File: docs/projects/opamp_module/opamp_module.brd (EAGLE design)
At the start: 58.1 x 25.4 mm, 12 parts, among them IC1 TL071P, IC2 TL072P

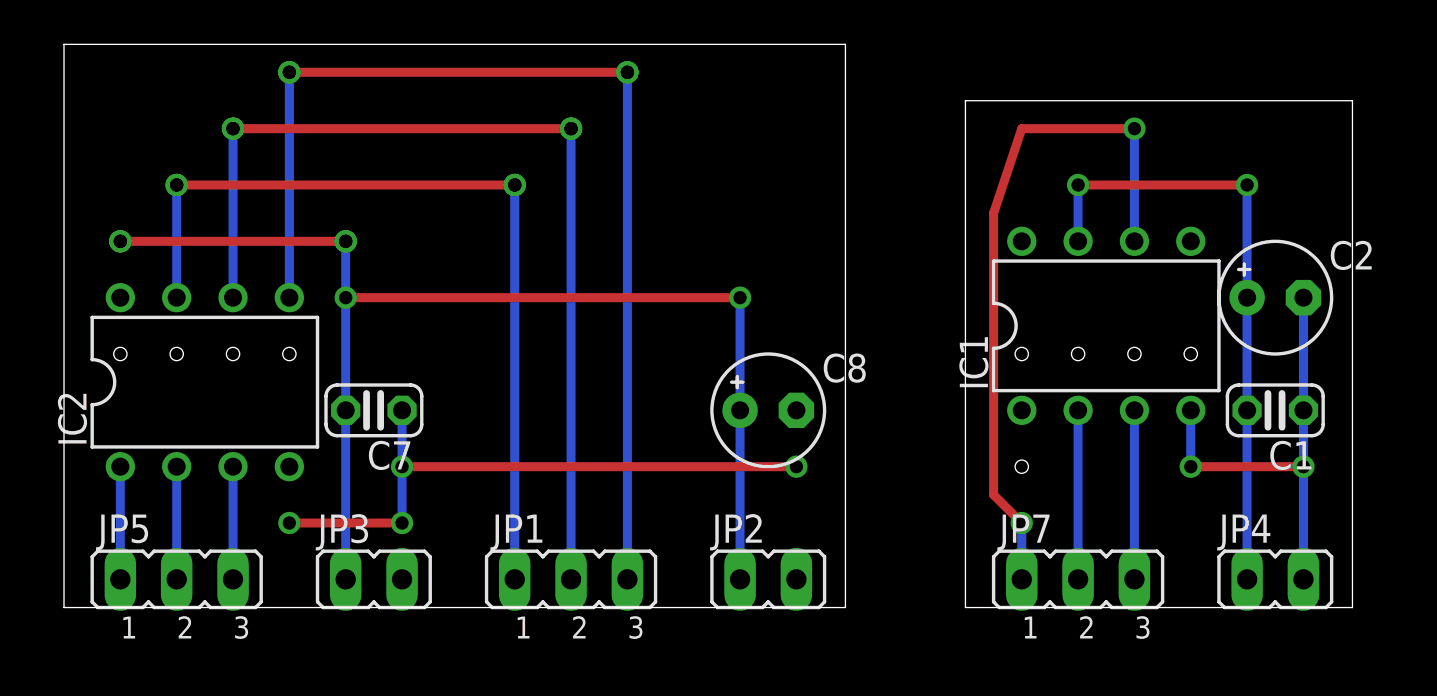
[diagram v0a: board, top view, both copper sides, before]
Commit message: fix airwires
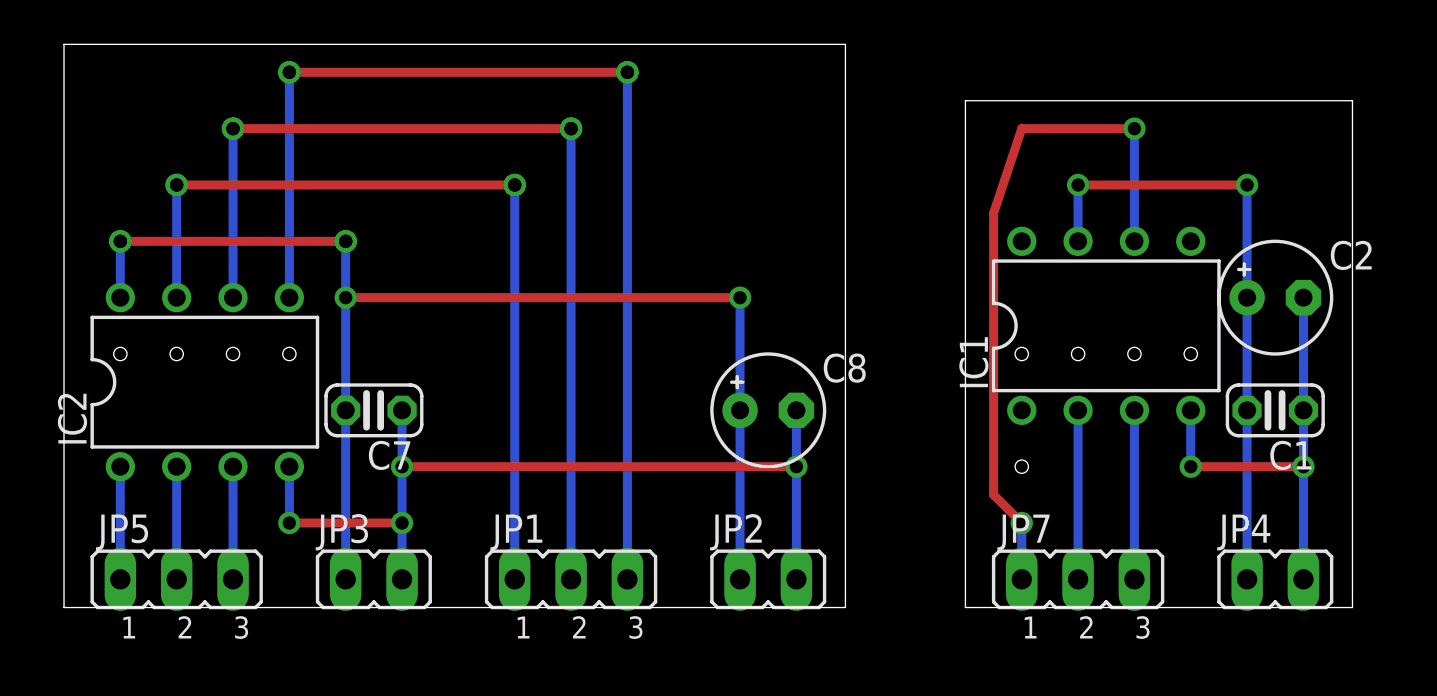
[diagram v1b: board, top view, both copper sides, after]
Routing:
- net N$2: track 27.9 -> 40.6 mm
- net N$8: track 55.9 -> 58.4 mm
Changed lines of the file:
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@@
 <grid distance="0.1" unitdist="inch" unit="inch" style="dots" multiple="1" display="yes" altdistance="0.05" altunitdist="inch" altunit="inch"/>
 <layers>
-<layer number="1" name="Top" color="4" fill="1" visible="no" active="yes"/>
-<layer number="16" name="Bottom" color="1" fill="1" visible="no" active="yes"/>
-<layer number="17" name="Pads" color="2" fill="1" visible="no" active="yes"/>
-<layer number="18" name="Vias" color="2" fill="1" visible="no" active="yes"/>
-<layer number="19" name="Unrouted" color="6" fill="1" visible="no" active="yes"/>
-<layer number="20" name="Dimension" color="15" fill="1" visible="no" active="yes"/>
-<layer number="21" name="tPlace" color="7" fill="1" visible="no" active="yes"/>
-<layer number="22" name="bPlace" color="7" fill="1" visible="no" active="yes"/>
-<layer number="23" name="tOrigins" color="15" fill="1" visible="no" active="yes"/>
-<layer number="24" name="bOrigins" color="15" fill="1" visible="no" active="yes"/>
-<layer number="25" name="tNames" color="7" fill="1" visible="no" active="yes"/>
-<layer number="26" name="bNames" color="7" fill="1" visible="no" active="yes"/>
-<layer number="27" name="tValues" color="7" fill="1" visible="no" active="yes"/>
-<layer number="28" name="bValues" color="7" fill="1" visible="no" active="yes"/>
-<layer number="29" name="tStop" color="7" fill="3" visible="no" active="yes"/>
-<layer number="30" name="bStop" color="7" fill="6" visible="no" active="yes"/>
-<layer number="31" name="tCream" color="7" fill="4" visible="no" active="yes"/>
-<layer number="32" name="bCream" color="7" fill="5" visible="no" active="yes"/>
-<layer number="33" name="tFinish" color="6" fill="3" visible="no" active="yes"/>
-<layer number="34" name="bFinish" color="6" fill="6" visible="no" active="yes"/>
-<layer number="35" name="tGlue" color="7" fill="4" visible="no" active="yes"/>
-<layer number="36" name="bGlue" color="7" fill="5" visible="no" active="yes"/>
-<layer number="37" name="tTest" color="7" fill="1" visible="no" active="yes"/>
-<layer number="38" name="bTest" color="7" fill="1" visible="no" active="yes"/>
-<layer number="39" name="tKeepout" color="4" fill="11" visible="no" active="yes"/>
-<layer number="40" name="bKeepout" color="1" fill="11" visible="no" active="yes"/>
-<layer number="41" name="tRestrict" color="4" fill="10" visible="no" active="yes"/>
-<layer number="42" name="bRestrict" color="1" fill="10" visible="no" active="yes"/>
-<layer number="43" name="vRestrict" color="2" fill="10" visible="no" active="yes"/>
-<layer number="44" name="Drills" color="7" fill="1" visible="no" active="yes"/>
-<layer number="45" name="Holes" color="7" fill="1" visible="no" active="yes"/>
-<layer number="46" name="Milling" color="3" fill="1" visible="no" active="yes"/>
-<layer number="47" name="Measures" color="7" fill="1" visible="no" active="yes"/>
-<layer number="48" name="Document" color="7" fill="1" visible="no" active="yes"/>
-<layer number="49" name="Reference" color="7" fill="1" visible="no" active="yes"/>
-<layer number="50" name="dxf" color="7" fill="1" visible="no" active="yes"/>
-<layer number="51" name="tDocu" color="7" fill="1" visible="no" active="yes"/>
-<layer number="52" name="bDocu" color="7" fill="1" visible="no" active="yes"/>
+<layer number="1" name="Top" color="4" fill="1" visible="yes" active="yes"/>
+<layer number="16" name="Bottom" color="1" fill="1" visible="yes" active="yes"/>
+<layer number="17" name="Pads" color="2" fill="1" visible="yes" active="yes"/>
+<layer number="18" name="Vias" color="2" fill="1" visible="yes" active="yes"/>
+<layer number="19" name="Unrouted" color="6" fill="1" visible="yes" active="yes"/>
+<layer number="20" name="Dimension" color="15" fill="1" visible="yes" active="yes"/>
+<layer number="21" name="tPlace" color="7" fill="1" visible="yes" active="yes"/>
+<layer number="22" name="bPlace" color="7" fill="1" visible="yes" active="yes"/>
+<layer number="23" name="tOrigins" color="15" fill="1" visible="yes" active="yes"/>
+<layer number="24" name="bOrigins" color="15" fill="1" visible="yes" active="yes"/>
+<layer number="25" name="tNames" color="7" fill="1" visible="yes" active="yes"/>
+<layer number="26" name="bNames" color="7" fill="1" visible="yes" active="yes"/>
+<layer number="27" name="tValues" color="7" fill="1" visible="yes" active="yes"/>
+<layer number="28" name="bValues" color="7" fill="1" visible="yes" active="yes"/>
+<layer number="29" name="tStop" color="7" fill="3" visible="yes" active="yes"/>
+<layer number="30" name="bStop" color="7" fill="6" visible="yes" active="yes"/>
+<layer number="31" name="tCream" color="7" fill="4" visible="yes" active="yes"/>
+<layer number="32" name="bCream" color="7" fill="5" visible="yes" active="yes"/>
+<layer number="33" name="tFinish" color="6" fill="3" visible="yes" active="yes"/>
+<layer number="34" name="bFinish" color="6" fill="6" visible="yes" active="yes"/>
+<layer number="35" name="tGlue" color="7" fill="4" visible="yes" active="yes"/>
+<layer number="36" name="bGlue" color="7" fill="5" visible="yes" active="yes"/>
+<layer number="37" name="tTest" color="7" fill="1" visible="yes" active="yes"/>
+<layer number="38" name="bTest" color="7" fill="1" visible="yes" active="yes"/>
+<layer number="39" name="tKeepout" color="4" fill="11" visible="yes" active="yes"/>
+<layer number="40" name="bKeepout" color="1" fill="11" visible="yes" active="yes"/>
+<layer number="41" name="tRestrict" color="4" fill="10" visible="yes" active="yes"/>
+<layer number="42" name="bRestrict" color="1" fill="10" visible="yes" active="yes"/>
+<layer number="43" name="vRestrict" color="2" fill="10" visible="yes" active="yes"/>
+<layer number="44" name="Drills" color="7" fill="1" visible="yes" active="yes"/>
+<layer number="45" name="Holes" color="7" fill="1" visible="yes" active="yes"/>
+<layer number="46" name="Milling" color="3" fill="1" visible="yes" active="yes"/>
+<layer number="47" name="Measures" color="7" fill="1" visible="yes" active="yes"/>
+<layer number="48" name="Document" color="7" fill="1" visible="yes" active="yes"/>
+<layer number="49" name="Reference" color="7" fill="1" visible="yes" active="yes"/>
+<layer number="50" name="dxf" color="7" fill="1" visible="yes" active="yes"/>
+<layer number="51" name="tDocu" color="7" fill="1" visible="yes" active="yes"/>
+<layer number="52" name="bDocu" color="7" fill="1" visible="yes" active="yes"/>
 <layer number="91" name="Nets" color="2" fill="1" visible="no" active="no"/>
 <layer number="92" name="Busses" color="1" fill="1" visible="no" active="no"/>
@@
 <layer number="97" name="Info" color="7" fill="1" visible="no" active="no"/>
 <layer number="98" name="Guide" color="6" fill="1" visible="no" active="no"/>
-<layer number="101" name="Hidden" color="15" fill="1" visible="no" active="yes"/>
-<layer number="102" name="Changes" color="12" fill="1" visible="no" active="yes"/>
+<layer number="101" name="Hidden" color="15" fill="1" visible="yes" active="yes"/>
+<layer number="102" name="Changes" color="12" fill="1" visible="yes" active="yes"/>
 <layer number="110" name="doc_red" color="4" fill="1" visible="yes" active="yes"/>
 <layer number="111" name="doc_blue" color="1" fill="1" visible="yes" active="yes"/>
@@
 <wire x1="35.56" y1="15.24" x2="35.56" y2="10.16" width="0.4064" layer="16"/>
 <wire x1="17.78" y1="15.24" x2="35.56" y2="15.24" width="0.4064" layer="1"/>
-<wire x1="7.62" y1="17.78" x2="7.62" y2="15.24" width="0" layer="19" extent="1-1"/>
 <via x="17.78" y="17.78" extent="1-16" drill="0.6" shape="square"/>
 <via x="17.78" y="15.24" extent="1-16" drill="0.6" shape="square"/>
@@
 <via x="17.78" y="17.78" extent="1-16" drill="0.6" shape="square"/>
 <via x="35.56" y="15.24" extent="1-16" drill="0.6" shape="square"/>
+<wire x1="7.62" y1="17.78" x2="7.62" y2="15.24" width="0.4064" layer="16"/>
 </signal>
 <signal name="N$9">
@@
 <wire x1="15.24" y1="5.08" x2="20.32" y2="5.08" width="0.4064" layer="1"/>
 <wire x1="20.32" y1="7.62" x2="38.1" y2="7.62" width="0.4064" layer="1"/>
-<wire x1="38.1" y1="7.62" x2="38.1" y2="10.16" width="0" layer="19" extent="1-1"/>
-<wire x1="15.24" y1="7.62" x2="15.24" y2="5.08" width="0" layer="19" extent="1-1"/>
-<wire x1="20.32" y1="2.54" x2="20.32" y2="5.08" width="0" layer="19" extent="16-16"/>
-<wire x1="38.1" y1="2.54" x2="38.1" y2="7.62" width="0" layer="19" extent="1-1"/>
 <via x="20.32" y="5.08" extent="1-16" drill="0.6" shape="square"/>
 <via x="20.32" y="7.62" extent="1-16" drill="0.6" shape="square"/>
 <via x="38.1" y="7.62" extent="1-16" drill="0.6" shape="square"/>
 <via x="15.24" y="5.08" extent="1-16" drill="0.6" shape="square"/>
+<wire x1="38.1" y1="2.54" x2="38.1" y2="7.62" width="0.4064" layer="16"/>
+<wire x1="15.24" y1="5.08" x2="15.24" y2="7.62" width="0.4064" layer="16"/>
+<wire x1="38.1" y1="7.62" x2="38.1" y2="10.16" width="0.4064" layer="16"/>
+<wire x1="20.32" y1="2.54" x2="20.32" y2="5.08" width="0.4064" layer="16"/>
 </signal>
 </signals>
